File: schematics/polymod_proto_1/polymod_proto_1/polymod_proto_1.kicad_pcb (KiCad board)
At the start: 2 copper layers, 133 parts, among them J1 Conn_01x02_Male, J10 Conn_01x08_Male, J11 Conn_01x08_Male, J12 Conn_01x08_Male, J13 Conn_01x08_Male, J14 Conn_01x03_Male, J2 Conn_01x03_Male, J3 Conn_01x02_Male, J4 Barrel_Jack, J6 Conn_01x08_Male, J7 Conn_01x08_Male, J8 Conn_01x08_Male, J9 Conn_01x08_Male, SW1 SW_Push, SW2 SW_Push, SW3 SW_Push, SW4 SW_Push, U1 6N138, U10 74HC595, U11 74LS165, U12 74LS165, U13 74LS165, U2 74HC595, U3 74LS165, U4 4051, U5 74HC595, U6 74LS165, U7 4051, U8 74HC595, U9 74HC595

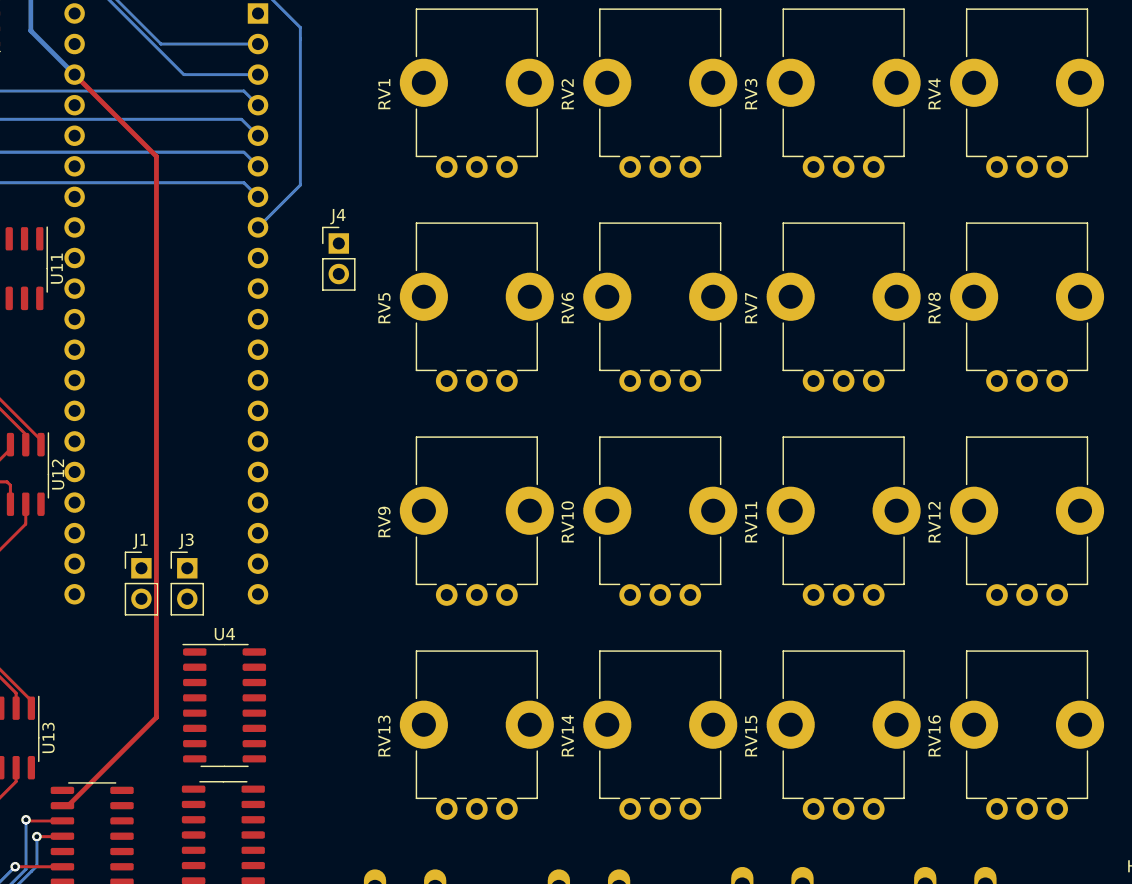
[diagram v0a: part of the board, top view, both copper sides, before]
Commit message: ummm less sure this is working well but not awful
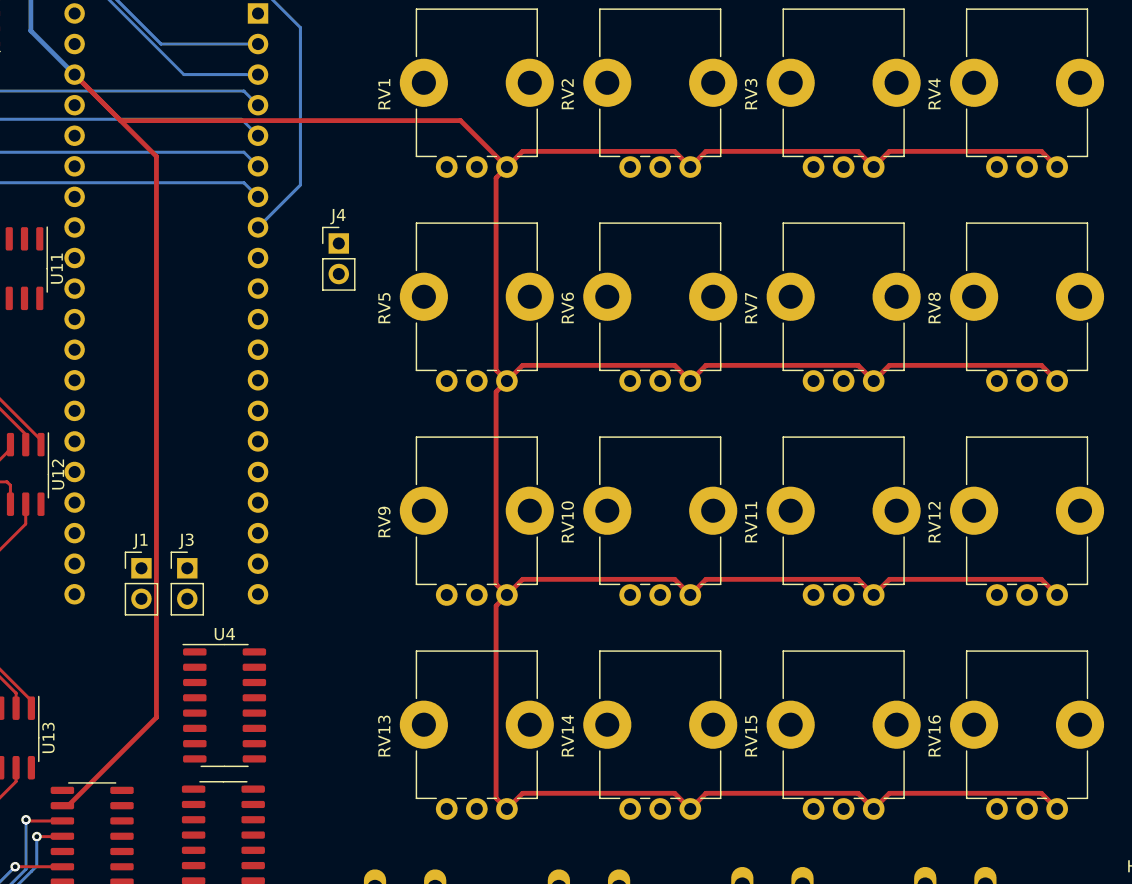
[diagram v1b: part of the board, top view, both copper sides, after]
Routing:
- net VCC: track 217.0 -> 507.5 mm
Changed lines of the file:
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@@
   )
   (segment (start 125.625 126.725) (end 126.107138 126.725) (width 0.4) (layer "F.Cu") (net 3))
+  (segment (start 206.980489 107.920489) (end 208.28 109.22) (width 0.4) (layer "F.Cu") (net 3))
+  (segment (start 191.740489 107.920489) (end 193.04 109.22) (width 0.4) (layer "F.Cu") (net 3))
+  (segment (start 162.56 109.22) (end 163.859511 107.920489) (width 0.4) (layer "F.Cu") (net 3))
   (segment (start 87.225 55.625) (end 85.275 55.625) (width 0.25) (layer "F.Cu") (net 3))
+  (segment (start 206.980489 72.360489) (end 208.28 73.66) (width 0.4) (layer "F.Cu") (net 3))
+  (segment (start 177.8 73.66) (end 179.099511 72.360489) (width 0.4) (layer "F.Cu") (net 3))
+  (segment (start 161.66 110.12) (end 161.66 126.1) (width 0.4) (layer "F.Cu") (net 3))
+  (segment (start 163.859511 107.920489) (end 176.500489 107.920489) (width 0.4) (layer "F.Cu") (net 3))
+  (segment (start 176.500489 107.920489) (end 177.8 109.22) (width 0.4) (layer "F.Cu") (net 3))
   (segment (start 87.025 77.825) (end 85.225 77.825) (width 0.4) (layer "F.Cu") (net 3))
+  (segment (start 191.740489 72.360489) (end 193.04 73.66) (width 0.4) (layer "F.Cu") (net 3))
+  (segment (start 206.980489 125.700489) (end 208.28 127) (width 0.4) (layer "F.Cu") (net 3))
+  (segment (start 161.66 74.56) (end 161.66 90.54) (width 0.4) (layer "F.Cu") (net 3))
+  (segment (start 162.56 109.22) (end 161.66 110.12) (width 0.4) (layer "F.Cu") (net 3))
   (segment (start 85.245 63.245) (end 85.2 63.2) (width 0.25) (layer "F.Cu") (net 3))
   (segment (start 87.025 100.975) (end 85.225 100.975) (width 0.4) (layer "F.Cu") (net 3))
   (segment (start 87.025 108.595) (end 85.295 108.595) (width 0.4) (layer "F.Cu") (net 3))
+  (segment (start 194.339511 72.360489) (end 206.980489 72.360489) (width 0.4) (layer "F.Cu") (net 3))
+  (segment (start 161.66 126.1) (end 162.56 127) (width 0.4) (layer "F.Cu") (net 3))
   (segment (start 85.355 85.445) (end 85.2 85.6) (width 0.4) (layer "F.Cu") (net 3))
+  (segment (start 162.56 127) (end 163.859511 125.700489) (width 0.4) (layer "F.Cu") (net 3))
+  (segment (start 194.339511 107.920489) (end 206.980489 107.920489) (width 0.4) (layer "F.Cu") (net 3))
+  (segment (start 179.099511 107.920489) (end 191.740489 107.920489) (width 0.4) (layer "F.Cu") (net 3))
   (segment (start 86.98 129.1) (end 87.025 129.145) (width 0.4) (layer "F.Cu") (net 3))
   (segment (start 85.225 100.975) (end 85.2 101) (width 0.4) (layer "F.Cu") (net 3))
+  (segment (start 162.56 91.44) (end 163.859511 90.140489) (width 0.4) (layer "F.Cu") (net 3))
+  (segment (start 162.56 73.66) (end 163.859511 72.360489) (width 0.4) (layer "F.Cu") (net 3))
+  (segment (start 179.099511 72.360489) (end 191.740489 72.360489) (width 0.4) (layer "F.Cu") (net 3))
+  (segment (start 177.8 109.22) (end 179.099511 107.920489) (width 0.4) (layer "F.Cu") (net 3))
+  (segment (start 176.500489 72.360489) (end 177.8 73.66) (width 0.4) (layer "F.Cu") (net 3))
+  (segment (start 163.859511 90.140489) (end 176.500489 90.140489) (width 0.4) (layer "F.Cu") (net 3))
+  (segment (start 193.04 127) (end 194.339511 125.700489) (width 0.4) (layer "F.Cu") (net 3))
   (segment (start 85.275 55.625) (end 85.2 55.7) (width 0.25) (layer "F.Cu") (net 3))
+  (segment (start 206.980489 90.140489) (end 208.28 91.44) (width 0.4) (layer "F.Cu") (net 3))
   (segment (start 87.025 129.145) (end 85.245 129.145) (width 0.4) (layer "F.Cu") (net 3))
   (segment (start 133.439511 72.782011) (end 126.6375 65.98) (width 0.4) (layer "F.Cu") (net 3))
+  (segment (start 191.740489 125.700489) (end 193.04 127) (width 0.4) (layer "F.Cu") (net 3))
+  (segment (start 177.8 127) (end 179.099511 125.700489) (width 0.4) (layer "F.Cu") (net 3))
   (segment (start 87.025 85.445) (end 85.355 85.445) (width 0.4) (layer "F.Cu") (net 3))
+  (segment (start 191.740489 90.140489) (end 193.04 91.44) (width 0.4) (layer "F.Cu") (net 3))
+  (segment (start 193.04 109.22) (end 194.339511 107.920489) (width 0.4) (layer "F.Cu") (net 3))
   (segment (start 85.225 77.825) (end 85.2 77.8) (width 0.4) (layer "F.Cu") (net 3))
+  (segment (start 176.500489 125.700489) (end 177.8 127) (width 0.4) (layer "F.Cu") (net 3))
   (segment (start 85.225 121.525) (end 85.2 121.5) (width 0.4) (layer "F.Cu") (net 3))
+  (segment (start 130.4575 69.8) (end 158.7 69.8) (width 0.4) (layer "F.Cu") (net 3))
+  (segment (start 162.56 91.44) (end 161.66 92.34) (width 0.4) (layer "F.Cu") (net 3))
+  (segment (start 193.04 91.44) (end 194.339511 90.140489) (width 0.4) (layer "F.Cu") (net 3))
   (segment (start 85.245 129.145) (end 85.2 129.1) (width 0.4) (layer "F.Cu") (net 3))
+  (segment (start 161.66 92.34) (end 161.66 108.32) (width 0.4) (layer "F.Cu") (net 3))
+  (segment (start 163.859511 125.700489) (end 176.500489 125.700489) (width 0.4) (layer "F.Cu") (net 3))
+  (segment (start 158.7 69.8) (end 162.56 73.66) (width 0.4) (layer "F.Cu") (net 3))
   (segment (start 85.295 108.595) (end 85.2 108.5) (width 0.4) (layer "F.Cu") (net 3))
   (segment (start 87.225 63.245) (end 85.245 63.245) (width 0.25) (layer "F.Cu") (net 3))
+  (segment (start 179.099511 90.140489) (end 191.740489 90.140489) (width 0.4) (layer "F.Cu") (net 3))
+  (segment (start 177.8 91.44) (end 179.099511 90.140489) (width 0.4) (layer "F.Cu") (net 3))
+  (segment (start 179.099511 125.700489) (end 191.740489 125.700489) (width 0.4) (layer "F.Cu") (net 3))
+  (segment (start 126.6375 65.98) (end 130.4575 69.8) (width 0.4) (layer "F.Cu") (net 3))
   (segment (start 126.107138 126.725) (end 133.439511 119.392627) (width 0.4) (layer "F.Cu") (net 3))
+  (segment (start 176.500489 90.140489) (end 177.8 91.44) (width 0.4) (layer "F.Cu") (net 3))
   (segment (start 133.439511 119.392627) (end 133.439511 72.782011) (width 0.4) (layer "F.Cu") (net 3))
+  (segment (start 162.56 73.66) (end 161.66 74.56) (width 0.4) (layer "F.Cu") (net 3))
+  (segment (start 194.339511 90.140489) (end 206.980489 90.140489) (width 0.4) (layer "F.Cu") (net 3))
   (segment (start 87.025 121.525) (end 85.225 121.525) (width 0.4) (layer "F.Cu") (net 3))
+  (segment (start 194.339511 125.700489) (end 206.980489 125.700489) (width 0.4) (layer "F.Cu") (net 3))
+  (segment (start 161.66 90.54) (end 162.56 91.44) (width 0.4) (layer "F.Cu") (net 3))
+  (segment (start 163.859511 72.360489) (end 176.500489 72.360489) (width 0.4) (layer "F.Cu") (net 3))
+  (segment (start 161.66 108.32) (end 162.56 109.22) (width 0.4) (layer "F.Cu") (net 3))
+  (segment (start 193.04 73.66) (end 194.339511 72.360489) (width 0.4) (layer "F.Cu") (net 3))
   (via (at 85.2 63.2) (size 0.8) (drill 0.4) (layers "F.Cu" "B.Cu") (net 3))
   (via (at 85.2 77.8) (size 0.8) (drill 0.4) (layers "F.Cu" "B.Cu") (net 3))
